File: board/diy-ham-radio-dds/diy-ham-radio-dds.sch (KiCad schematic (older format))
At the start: 63 parts, among them J1 ICSP, J2 I2C, J3 VCC, J4 NPN OUT, J5 , J6 UART_PROG, Q1 S0805, Q2 S0805, Q3 S0805, Q4 S0805, Q5 S0805, Q6 S0805, Q7 S0805, Q8 S0805, SW1 SW_Push, SW2 SW_Push, SW3 SW_Push, SW4 SW_Push, SW5 Rotary_Encoder_Switch, U1 ATmega328-AU, U2 74LS08, U3 L7805, U4 74HC595, Y1 16MHz

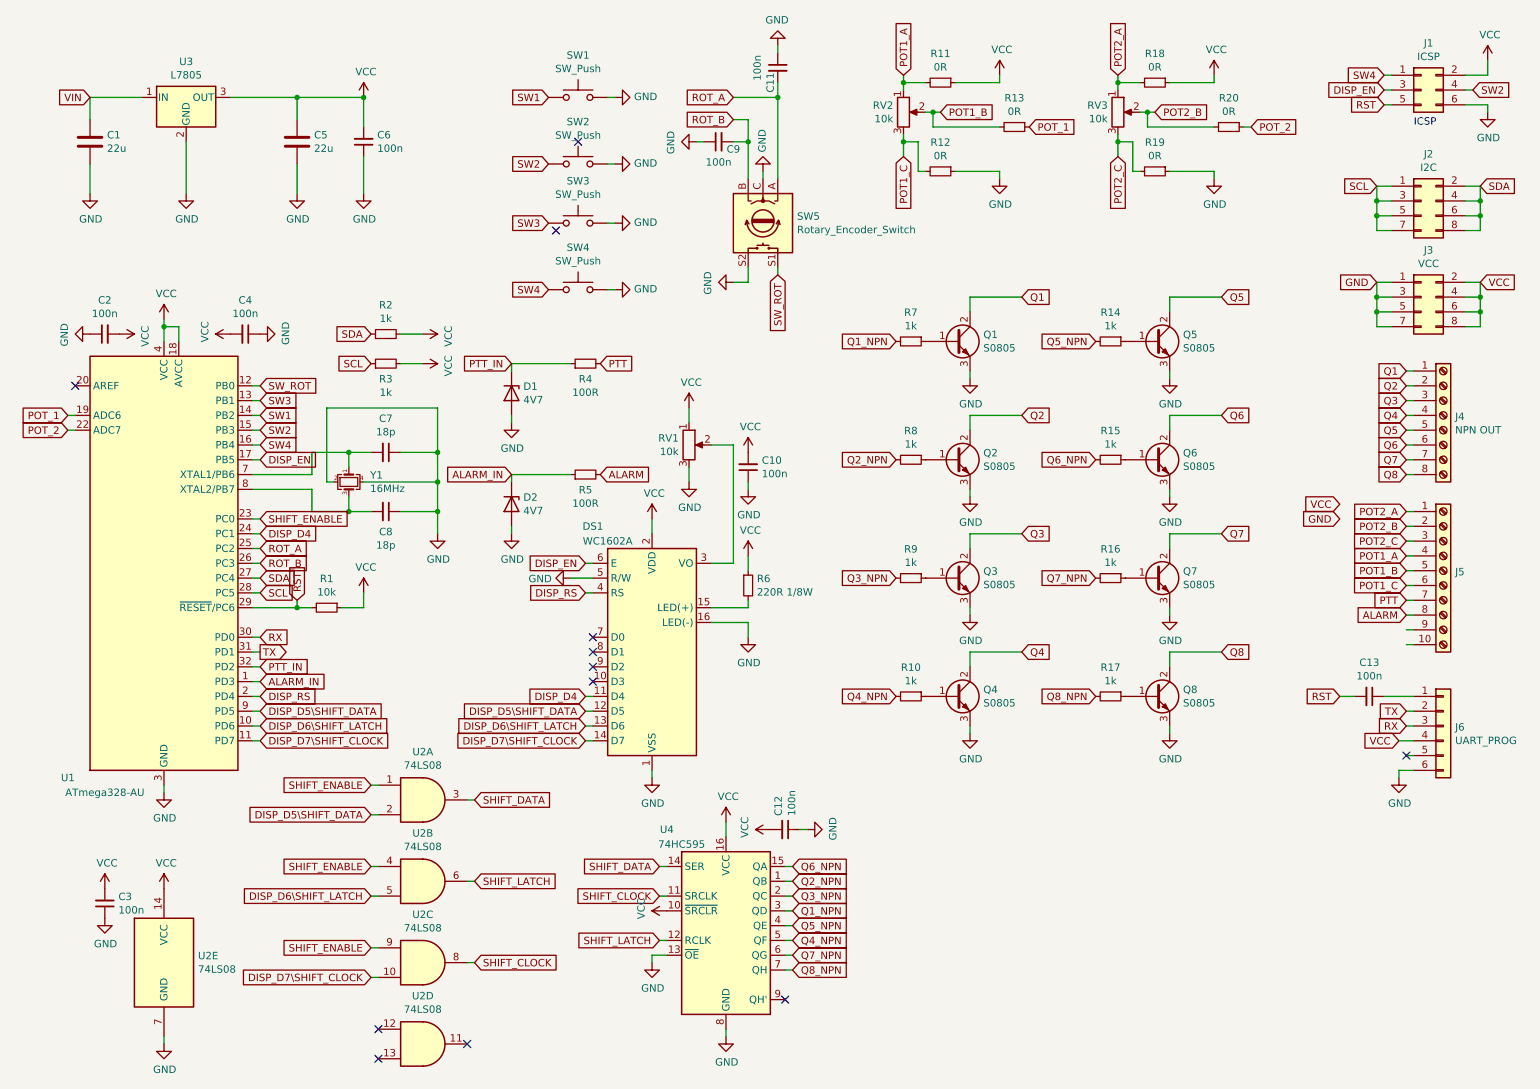
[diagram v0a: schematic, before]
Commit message: Finalised board drawing
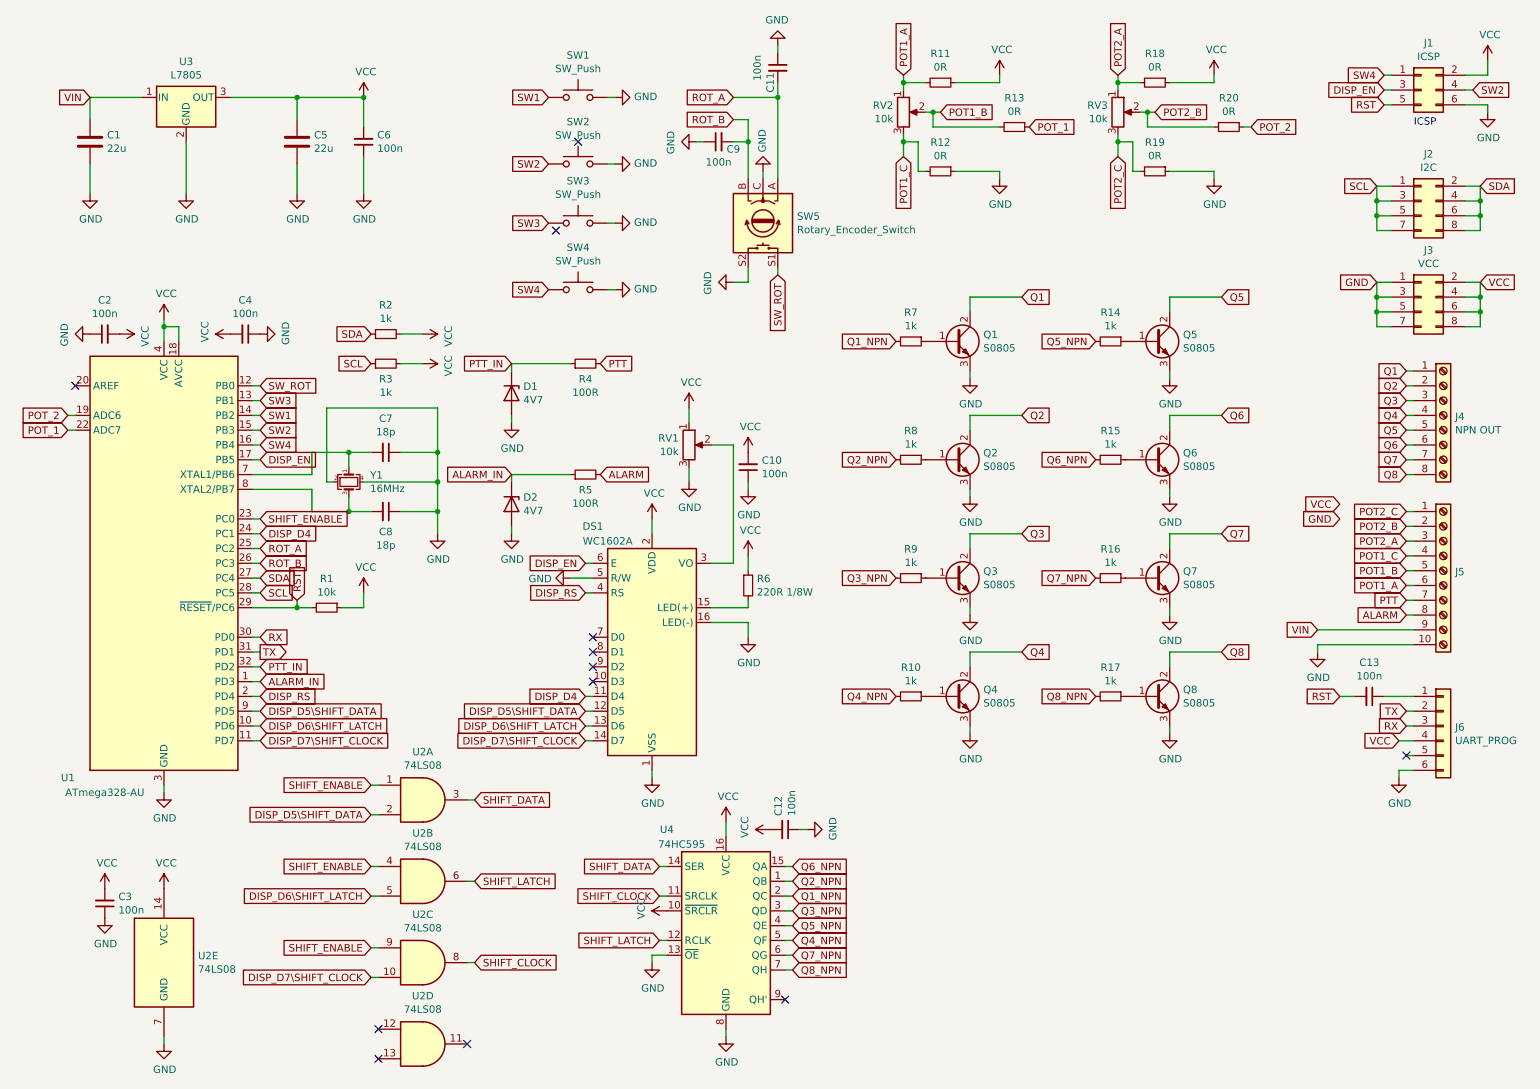
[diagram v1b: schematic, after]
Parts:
- J1: footprint Connector_PinHeader_1.00mm:PinHeader_2x03_P1.00mm_Vertical -> Connector_PinHeader_2.54mm:PinHeader_2x03_P2.54mm_Vertical
- J2, J3: footprint Connector_PinHeader_1.00mm:PinHeader_2x04_P1.00mm_Vertical -> Connector_PinHeader_2.54mm:PinHeader_2x04_P2.54mm_Vertical
- J6: footprint Connector_PinHeader_1.27mm:PinHeader_1x06_P1.27mm_Vertical -> Connector_PinHeader_2.54mm:PinHeader_1x06_P2.54mm_Vertical
- RV1: footprint Potentiometer_THT:Potentiometer_Alpha_RD901F-40-00D_Single_Vertical -> Potentiometer_THT:Potentiometer_Bourns_3296W_Vertical
- U3: footprint Package_TO_SOT_THT:TO-220-3_Vertical -> Package_TO_SOT_THT:TO-220-3_Horizontal_TabDown
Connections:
- net GND: now also J5.10 (Pin_10)
- net POT1_A: now also J5.6 (Pin_6); no longer J5.4 (Pin_4)
- net POT1_C: now also J5.4 (Pin_4); no longer J5.6 (Pin_6)
- net POT2_A: now also J5.3 (Pin_3); no longer J5.1 (Pin_1)
- net POT2_C: now also J5.1 (Pin_1); no longer J5.3 (Pin_3)
- net POT_1: now also U1.22 (ADC7); no longer U1.19 (ADC6)
- net POT_2: now also U1.19 (ADC6); no longer U1.22 (ADC7)
- net Q1_NPN: now also U4.2 (QC); no longer U4.3 (QD)
- net Q3_NPN: now also U4.3 (QD); no longer U4.2 (QC)
- net VIN: now also J5.9 (Pin_9)
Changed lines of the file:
@@
 F 0 "U3" H 1700 1392 50  0000 C CNN
 F 1 "L7805" H 1700 1301 50  0000 C CNN
-F 2 "Package_TO_SOT_THT:TO-220-3_Vertical" H 1725 1000 50  0001 L CIN
+F 2 "Package_TO_SOT_THT:TO-220-3_Horizontal_TabDown" H 1725 1000 50  0001 L CIN
 F 3 "http://www.st.com/content/ccc/resource/technical/document/datasheet/41/4f/b3/b0/12/d4/47/88/CD00000444.pdf/files/CD00000444.pdf/jcr:content/translations/en.CD00000444.pdf" H 1700 1100 50  0001 C CNN
 	1    1700 1150
@@
 F 0 "RV1" H 5030 3546 50  0000 R CNN
 F 1 "10k" H 5030 3455 50  0000 R CNN
-F 2 "Potentiometer_THT:Potentiometer_Alpha_RD901F-40-00D_Single_Vertical" H 5100 3500 50  0001 C CNN
+F 2 "Potentiometer_THT:Potentiometer_Bourns_3296W_Vertical" H 5100 3500 50  0001 C CNN
 F 3 "~" H 5100 3500 50  0001 C CNN
 	1    5100 3500
@@
 Text GLabel 2200 3500 2    50   Input ~ 0
 SW4
+Text GLabel 900  3400 0    50   Input ~ 0
+POT_1
 Text GLabel 900  3300 0    50   Input ~ 0
-POT_1
-Text GLabel 900  3400 0    50   Input ~ 0
 POT_2
 Text GLabel 2200 3100 2    50   Input ~ 0
@@
 F 0 "J1" H 10100 1417 50  0000 C CNN
 F 1 "ICSP" H 10100 1326 50  0000 C CNN
-F 2 "Connector_PinHeader_1.00mm:PinHeader_2x03_P1.00mm_Vertical" H 10050 1100 50  0001 C CNN
+F 2 "Connector_PinHeader_2.54mm:PinHeader_2x03_P2.54mm_Vertical" H 10050 1100 50  0001 C CNN
 F 3 "~" H 10050 1100 50  0001 C CNN
 	1    10050 1100
@@
 F 0 "J2" H 10100 2167 50  0000 C CNN
 F 1 "I2C" H 10100 2076 50  0000 C CNN
-F 2 "Connector_PinHeader_1.00mm:PinHeader_2x04_P1.00mm_Vertical" H 10050 1850 50  0001 C CNN
+F 2 "Connector_PinHeader_2.54mm:PinHeader_2x04_P2.54mm_Vertical" H 10050 1850 50  0001 C CNN
 F 3 "~" H 10050 1850 50  0001 C CNN
 	1    10050 1850
@@
 F 0 "J3" H 10100 2817 50  0000 C CNN
 F 1 "VCC" H 10100 2726 50  0000 C CNN
-F 2 "Connector_PinHeader_1.00mm:PinHeader_2x04_P1.00mm_Vertical" H 10050 2500 50  0001 C CNN
+F 2 "Connector_PinHeader_2.54mm:PinHeader_2x04_P2.54mm_Vertical" H 10050 2500 50  0001 C CNN
 F 3 "~" H 10050 2500 50  0001 C CNN
 	1    10050 2500
@@
 Text GLabel 9500 4000 0    50   Input ~ 0
 GND
-Text GLabel 9950 4250 0    50   Input ~ 0
-POT1_A
 Text GLabel 9950 4350 0    50   Input ~ 0
 POT1_B
-Text GLabel 9950 4450 0    50   Input ~ 0
-POT1_C
-Text GLabel 9950 3950 0    50   Input ~ 0
+Text GLabel 9950 4150 0    50   Input ~ 0
 POT2_A
 Text GLabel 9950 4050 0    50   Input ~ 0
 POT2_B
-Text GLabel 9950 4150 0    50   Input ~ 0
+Text GLabel 9950 3950 0    50   Input ~ 0
 POT2_C
 $Comp
@@
 Text GLabel 9950 4650 0    50   Input ~ 0
 ALARM
-Text GLabel 5800 6650 2    50   Input ~ 0
+Text GLabel 5800 6550 2    50   Input ~ 0
 Q1_NPN
 Text GLabel 5800 6450 2    50   Input ~ 0
 Q2_NPN
-Text GLabel 5800 6550 2    50   Input ~ 0
+Text GLabel 5800 6650 2    50   Input ~ 0
 Q3_NPN
 Text GLabel 5800 6850 2    50   Input ~ 0
@@
 	9950 4650 10000 4650
 Wire Wire Line
-	9950 4750 10000 4750
-Wire Wire Line
-	9950 4850 10000 4850
-Wire Wire Line
 	10350 1100 10400 1100
 Text GLabel 10400 1100 2    50   Input ~ 0
@@
 F 0 "J6" H 10280 5392 50  0000 L CNN
 F 1 "UART_PROG" H 10280 5301 50  0000 L CNN
-F 2 "Connector_PinHeader_1.27mm:PinHeader_1x06_P1.27mm_Vertical" H 10200 5400 50  0001 C CNN
+F 2 "Connector_PinHeader_2.54mm:PinHeader_1x06_P2.54mm_Vertical" H 10200 5400 50  0001 C CNN
 F 3 "~" H 10200 5400 50  0001 C CNN
 	1    10200 5400
@@
 NoConn ~ 4200 2050
 NoConn ~ 4350 1450
+$Comp
+L power:GND #PWR0101
+U 1 1 601EB40E
+P 9350 4900
+F 0 "#PWR0101" H 9350 4650 50  0001 C CNN
+F 1 "GND" H 9355 4727 50  0000 C CNN
+F 2 "" H 9350 4900 50  0001 C CNN
+F 3 "" H 9350 4900 50  0001 C CNN
+	1    9350 4900
+	1    0    0    -1
+$EndComp
+Text GLabel 9350 4750 0    50   Input ~ 0
+VIN
+Wire Wire Line
+	9350 4750 10000 4750
+Wire Wire Line
+	9350 4900 9350 4850
+Wire Wire Line
+	9350 4850 10000 4850
+Text GLabel 9950 4250 0    50   Input ~ 0
+POT1_C
+Text GLabel 9950 4450 0    50   Input ~ 0
+POT1_A
 $EndSCHEMATC
